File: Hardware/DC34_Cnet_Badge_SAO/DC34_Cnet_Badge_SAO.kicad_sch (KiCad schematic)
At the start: 4 parts, among them J1 Conn_02x03_Top_Bottom

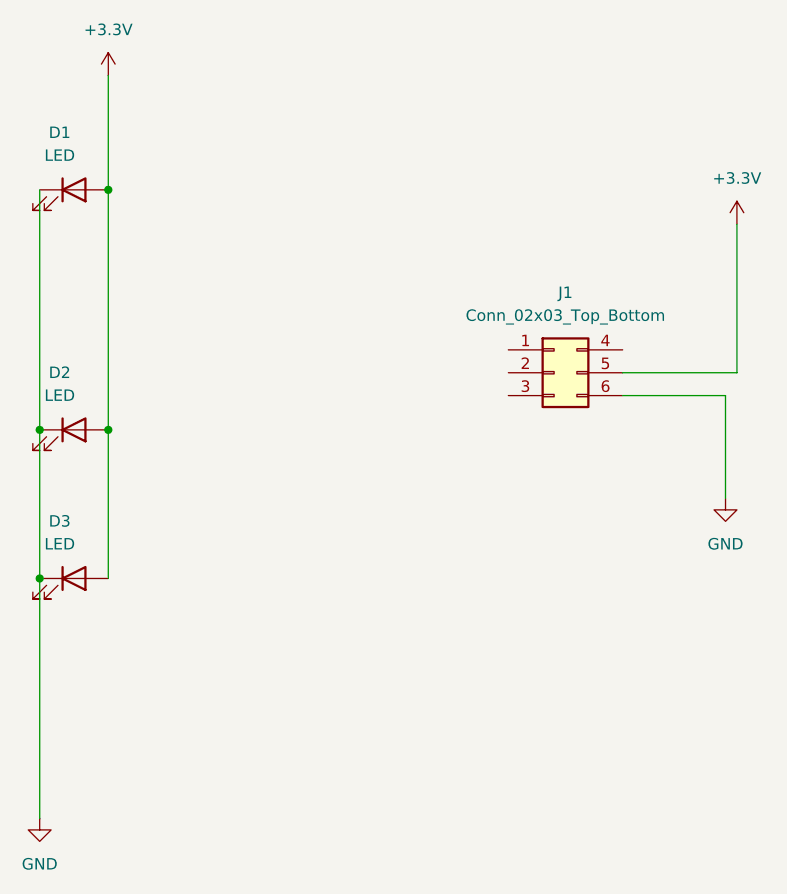
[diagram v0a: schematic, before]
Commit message: Updates
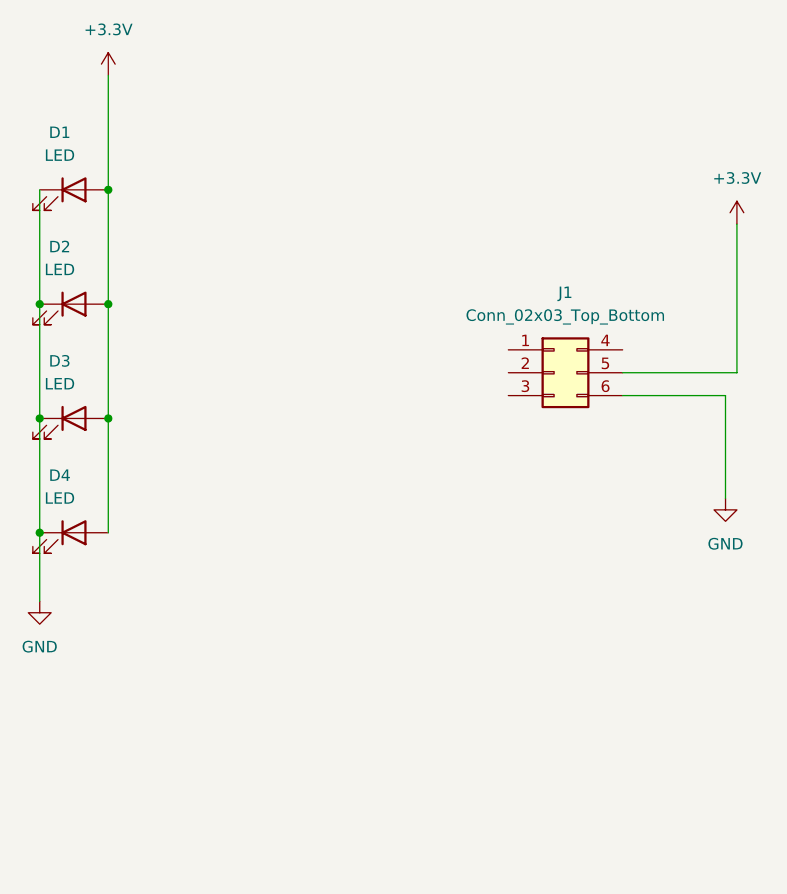
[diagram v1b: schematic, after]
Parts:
- added D4: LED, LED_THT:LED_D3.0mm, symbol Device:LED
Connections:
- net +3.3V: now also D4.2 (A)
- net GND: now also D4.1 (K)
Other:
- moved on the sheet: D2, D3
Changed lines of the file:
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@@
 	)
 	(junction
-		(at 80.01 90.17)
+		(at 80.01 88.9)
 		(diameter 0)
 		(color 0 0 0 0)
 	)
 	(junction
-		(at 87.63 90.17)
+		(at 87.63 88.9)
 		(diameter 0)
 		(color 0 0 0 0)
 	)
 	(junction
-		(at 80.01 106.68)
+		(at 87.63 76.2)
 		(diameter 0)
 		(color 0 0 0 0)
 	)
-	(wire
-		(pts
-			(xy 80.01 63.5) (xy 80.01 90.17)
-		)
-		(stroke
-			(width 0)
-			(type default)
-		)
-	)
-	(wire
-		(pts
-			(xy 87.63 63.5) (xy 87.63 90.17)
+	(junction
+		(at 80.01 101.6)
+		(diameter 0)
+		(color 0 0 0 0)
+	)
+	(junction
+		(at 80.01 76.2)
+		(diameter 0)
+		(color 0 0 0 0)
+	)
+	(wire
+		(pts
+			(xy 80.01 101.6) (xy 80.01 109.22)
+		)
+		(stroke
+			(width 0)
+			(type default)
+		)
+	)
+	(wire
+		(pts
+			(xy 87.63 76.2) (xy 87.63 88.9)
+		)
+		(stroke
+			(width 0)
+			(type default)
+		)
+	)
+	(wire
+		(pts
+			(xy 87.63 88.9) (xy 87.63 101.6)
+		)
+		(stroke
+			(width 0)
+			(type default)
+		)
+	)
+	(wire
+		(pts
+			(xy 80.01 63.5) (xy 80.01 76.2)
+		)
+		(stroke
+			(width 0)
+			(type default)
+		)
+	)
+	(wire
+		(pts
+			(xy 87.63 63.5) (xy 87.63 76.2)
+		)
+		(stroke
+			(width 0)
+			(type default)
+		)
+	)
+	(wire
+		(pts
+			(xy 80.01 88.9) (xy 80.01 101.6)
 		)
 		(stroke
@@
 	(wire
 		(pts
-			(xy 80.01 106.68) (xy 80.01 133.35)
-		)
-		(stroke
-			(width 0)
-			(type default)
-		)
-	)
-	(wire
-		(pts
-			(xy 80.01 90.17) (xy 80.01 106.68)
+			(xy 80.01 76.2) (xy 80.01 88.9)
 		)
 		(stroke
@@
 		(pts
 			(xy 157.48 67.31) (xy 157.48 83.82)
-		)
-		(stroke
-			(width 0)
-			(type default)
-		)
-	)
-	(wire
-		(pts
-			(xy 87.63 90.17) (xy 87.63 106.68)
 		)
 		(stroke
@@
 	(symbol
 		(lib_id "Device:LED")
-		(at 83.82 106.68 0)
+		(at 83.82 88.9 0)
 		(unit 1)
 		(exclude_from_sim no)
@@
 		(fields_autoplaced yes)
 		(property "Reference" "D3"
-			(at 82.2325 100.33 0)
+			(at 82.2325 82.55 0)
 			(effects
 				(font
@@
 		)
 		(property "Value" "LED"
-			(at 82.2325 102.87 0)
+			(at 82.2325 85.09 0)
 			(effects
 				(font
@@
 		)
 		(property "Footprint" "LED_THT:LED_D3.0mm"
-			(at 83.82 106.68 0)
+			(at 83.82 88.9 0)
 			(effects
 				(font
@@
 		)
 		(property "Datasheet" "~"
-			(at 83.82 106.68 0)
+			(at 83.82 88.9 0)
 			(effects
 				(font
@@
 		)
 		(property "Description" ""
-			(at 83.82 106.68 0)
+			(at 83.82 88.9 0)
 			(effects
 				(font
@@
 	(symbol
 		(lib_id "power:GND")
-		(at 80.01 133.35 0)
+		(at 80.01 109.22 0)
 		(unit 1)
 		(exclude_from_sim no)
@@
 		(fields_autoplaced yes)
 		(property "Reference" "#PWR0104"
-			(at 80.01 139.7 0)
+			(at 80.01 115.57 0)
 			(effects
 				(font
@@
 		)
 		(property "Value" "GND"
-			(at 80.01 138.43 0)
+			(at 80.01 114.3 0)
 			(effects
 				(font
@@
 		)
 		(property "Footprint" ""
-			(at 80.01 133.35 0)
+			(at 80.01 109.22 0)
 			(effects
 				(font
@@
 		)
 		(property "Datasheet" ""
-			(at 80.01 133.35 0)
+			(at 80.01 109.22 0)
 			(effects
 				(font
@@
 		)
 		(property "Description" ""
-			(at 80.01 133.35 0)
+			(at 80.01 109.22 0)
 			(effects
 				(font
@@
 	(symbol
 		(lib_id "Device:LED")
-		(at 83.82 90.17 0)
+		(at 83.82 76.2 0)
 		(unit 1)
 		(exclude_from_sim no)
@@
 		(fields_autoplaced yes)
 		(property "Reference" "D2"
-			(at 82.2325 83.82 0)
+			(at 82.2325 69.85 0)
 			(effects
 				(font
@@
 		)
 		(property "Value" "LED"
-			(at 82.2325 86.36 0)
+			(at 82.2325 72.39 0)
 			(effects
 				(font
@@
 		)
 		(property "Footprint" "LED_THT:LED_D3.0mm"
-			(at 83.82 90.17 0)
+			(at 83.82 76.2 0)
 			(effects
 				(font
@@
 		)
 		(property "Datasheet" "~"
-			(at 83.82 90.17 0)
+			(at 83.82 76.2 0)
 			(effects
 				(font
@@
 		)
 		(property "Description" ""
-			(at 83.82 90.17 0)
+			(at 83.82 76.2 0)
 			(effects
 				(font
@@
 					(unit 1)
 				)
+			)
+		)
+	)
+	(symbol
+		(lib_id "Device:LED")
+		(at 83.82 101.6 0)
+		(unit 1)
+		(exclude_from_sim no)
+		(in_bom yes)
+		(on_board yes)
+		(dnp no)
+		(fields_autoplaced yes)
+		(property "Reference" "D4"
+			(at 82.2325 95.25 0)
+			(effects
+				(font
+					(size 1.27 1.27)
+				)
+			)
+		)
+		(property "Value" "LED"
+			(at 82.2325 97.79 0)
+			(effects
+				(font
+					(size 1.27 1.27)
+				)
+			)
+		)
+		(property "Footprint" "LED_THT:LED_D3.0mm"
+			(at 83.82 101.6 0)
+			(effects
+				(font
+					(size 1.27 1.27)
+				)
+				(hide yes)
+			)
+		)
+		(property "Datasheet" "~"
+			(at 83.82 101.6 0)
+			(effects
+				(font
+					(size 1.27 1.27)
+				)
+				(hide yes)
+			)
+		)
+		(property "Description" ""
+			(at 83.82 101.6 0)
+			(effects
+				(font
+					(size 1.27 1.27)
+				)
+			)
+		)
+		(pin "1"
+		)
+		(pin "2"
+		)
+		(instances
+			(project "DC34_Cnet_Badge_SAO"
+				(path "/b082f5cf-66de-4c8b-a175-31df807e5ed7"
+					(reference "D4")
+					(unit 1)
+				)
